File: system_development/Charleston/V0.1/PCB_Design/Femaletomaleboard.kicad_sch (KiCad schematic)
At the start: 5 parts, among them J1 DB25_Receptacle, J2 Screw_Terminal_01x12, J3 Screw_Terminal_01x12

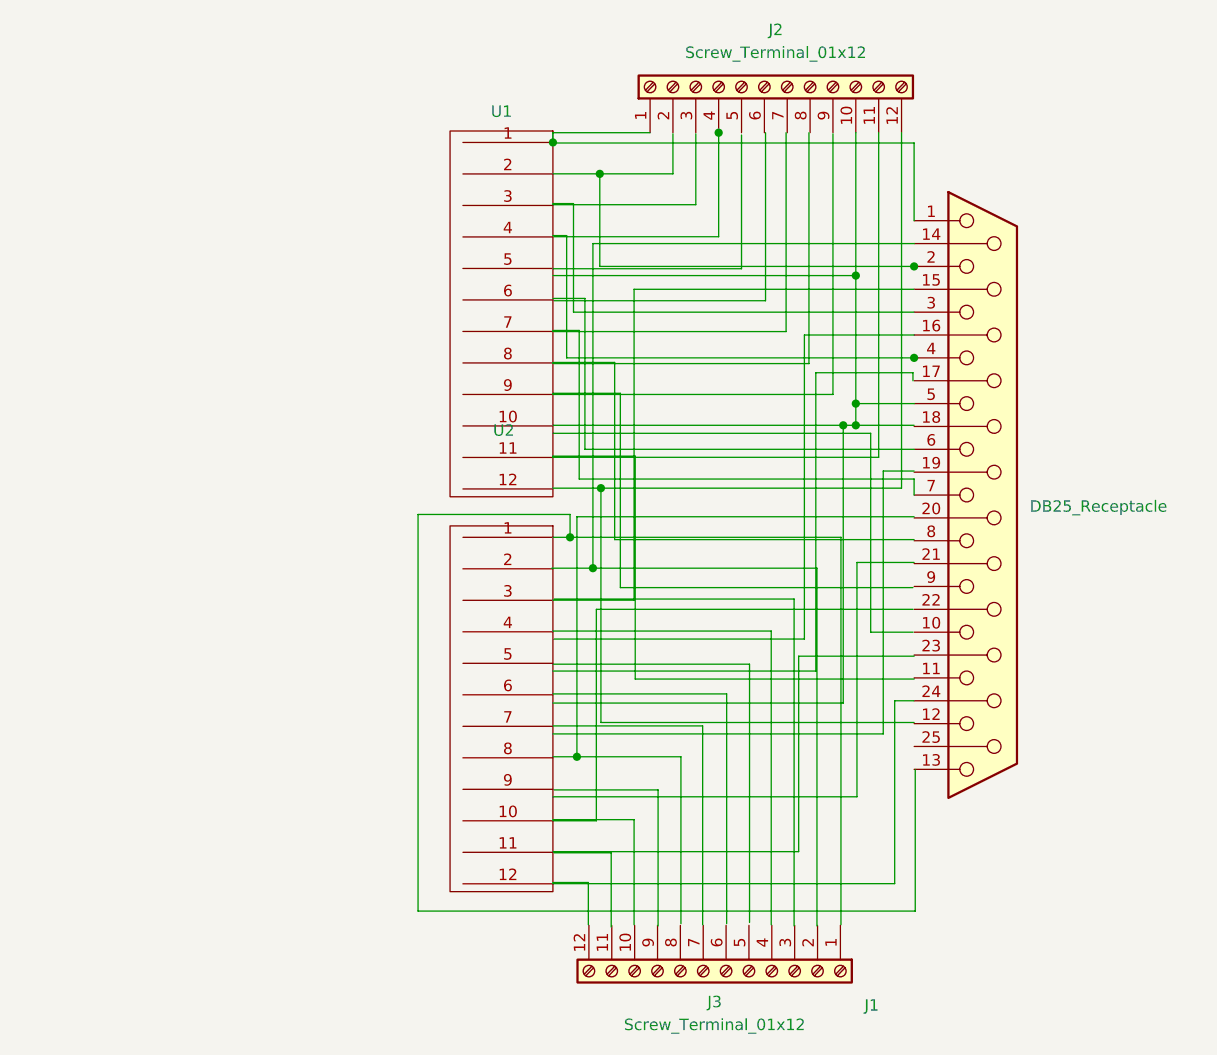
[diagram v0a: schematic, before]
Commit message: femaletomaleboard
4th times the charm
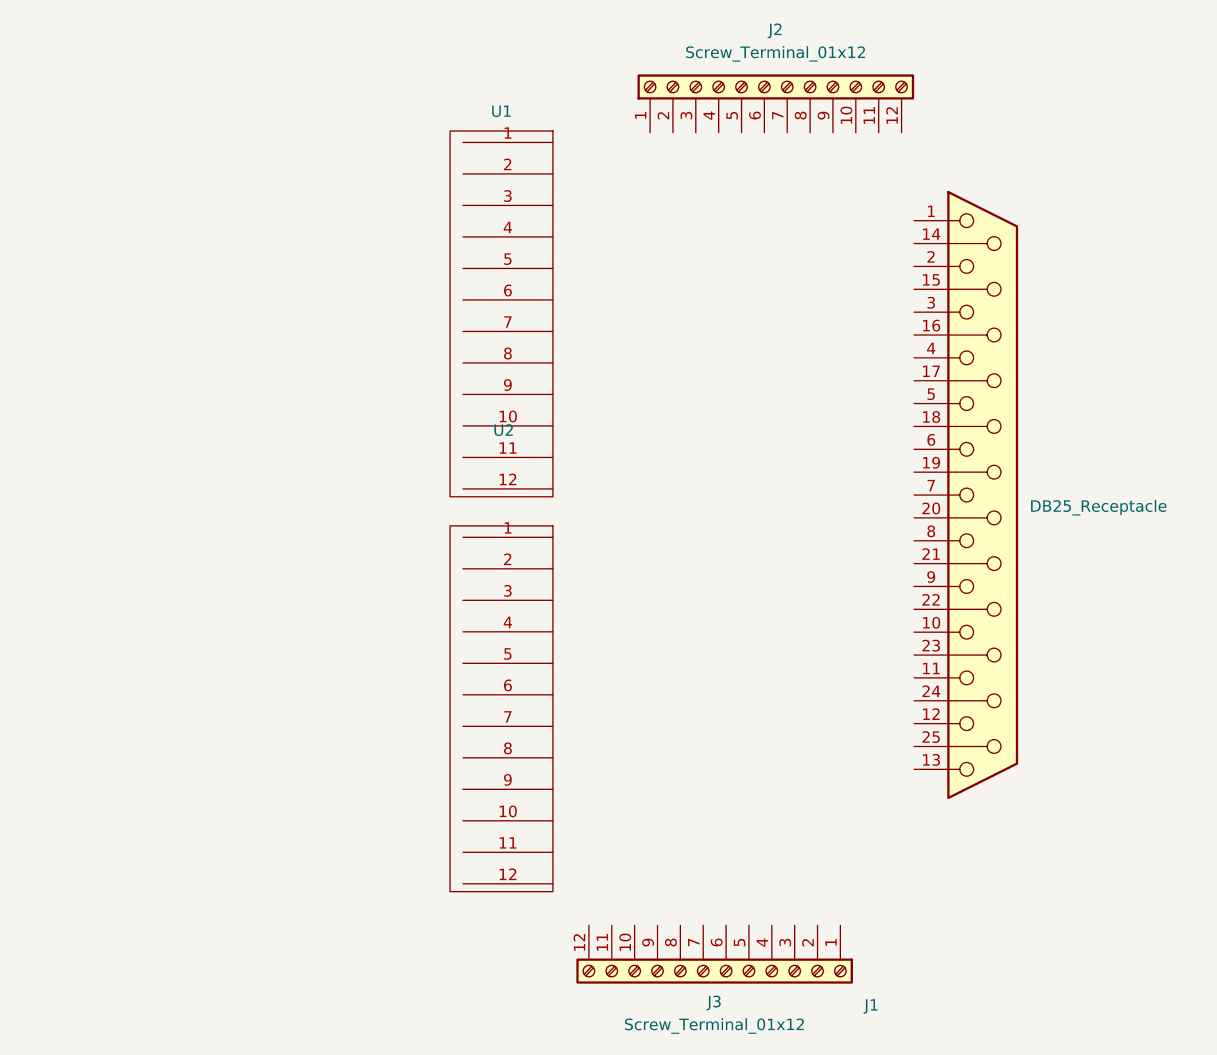
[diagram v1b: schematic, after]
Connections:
- net at J1.5: no longer J2.10 (Pin_10)
- now unconnected: J1.1, J2.1 (Pin_1), U1.1

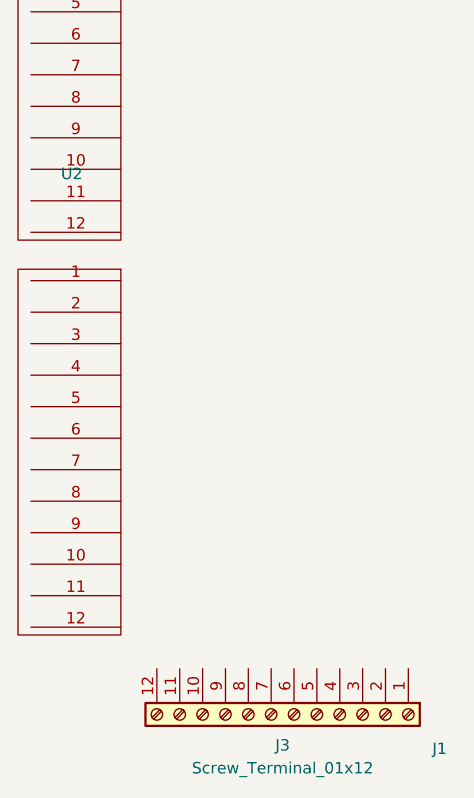
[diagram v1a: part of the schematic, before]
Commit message: updates
updates
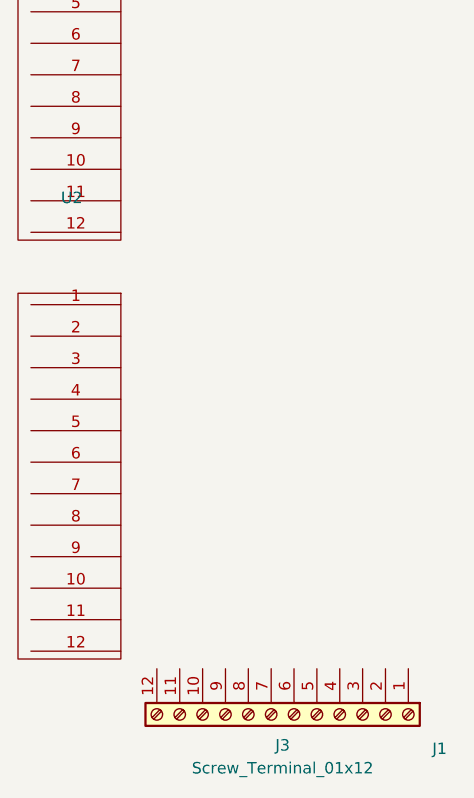
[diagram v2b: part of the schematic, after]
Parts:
- J1: symbol Connector:DB25_Receptacle -> libary_bms:DB25_Receptacle
- J2, J3: symbol Connector:Screw_Terminal_01x12 -> libary_bms:Screw_Terminal_01x12
- U1, U2: symbol Gold_Finger_connector:GoldFingerConnector -> libary_bms:GoldFingerConnector
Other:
- moved on the sheet: U2
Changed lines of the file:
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@@
 (kicad_sch (version 20230121) (generator eeschema)
   (paper "A4")
-  (symbol (lib_id "Connector:Screw_Terminal_01x12") (at 93.7895 114.7445 270) (unit 1)
+  (symbol (lib_id "libary_bms:Screw_Terminal_01x12") (at 93.7895 114.7445 270) (unit 1)
     (in_bom yes) (on_board yes) (dnp no) (fields_autoplaced)
     (property "Reference" "J3" (at 92.5195 118.1735 90)
@@
     )
   )
-  (symbol (lib_id "Gold_Finger_connector:GoldFingerConnector") (at 74.549 66.548 180) (unit 1)
+  (symbol (lib_id "libary_bms:GoldFingerConnector") (at 74.549 69.215 180) (unit 1)
     (in_bom yes) (on_board yes) (dnp no)
-    (property "Reference" "U2" (at 69.088 54.677 0)
+    (property "Reference" "U2" (at 69.088 57.344 0)
       (effects (font (size 1.27 1.27)))
     )
-    (property "Value" "~" (at 74.549 66.548 0)
+    (property "Value" "~" (at 74.549 69.215 0)
       (effects (font (size 1.27 1.27)))
     )
-    (property "Footprint" "" (at 74.549 66.548 0)
+    (property "Footprint" "" (at 74.549 69.215 0)
       (effects (font (size 1.27 1.27)) hide)
     )
-    (property "Datasheet" "" (at 74.549 66.548 0)
+    (property "Datasheet" "" (at 74.549 69.215 0)
       (effects (font (size 1.27 1.27)) hide)
     )
@@
     )
   )
-  (symbol (lib_id "Connector:DB25_Receptacle") (at 122.301 61.849 0) (unit 1)
+  (symbol (lib_id "libary_bms:DB25_Receptacle") (at 122.301 61.849 0) (unit 1)
     (in_bom yes) (on_board yes) (dnp no)
     (property "Reference" "J1" (at 109.1565 118.5545 0)
@@
     )
   )
-  (symbol (lib_id "Gold_Finger_connector:GoldFingerConnector") (at 74.549 22.673 180) (unit 1)
+  (symbol (lib_id "libary_bms:GoldFingerConnector") (at 74.549 22.673 180) (unit 1)
     (in_bom yes) (on_board yes) (dnp no)
     (property "Reference" "U1" (at 68.834 19.244 0)
@@
     )
   )
-  (symbol (lib_id "Connector:Screw_Terminal_01x12") (at 98.044 16.51 90) (unit 1)
+  (symbol (lib_id "libary_bms:Screw_Terminal_01x12") (at 98.044 16.51 90) (unit 1)
     (in_bom yes) (on_board yes) (dnp no) (fields_autoplaced)
     (property "Reference" "J2" (at 99.314 10.16 90)

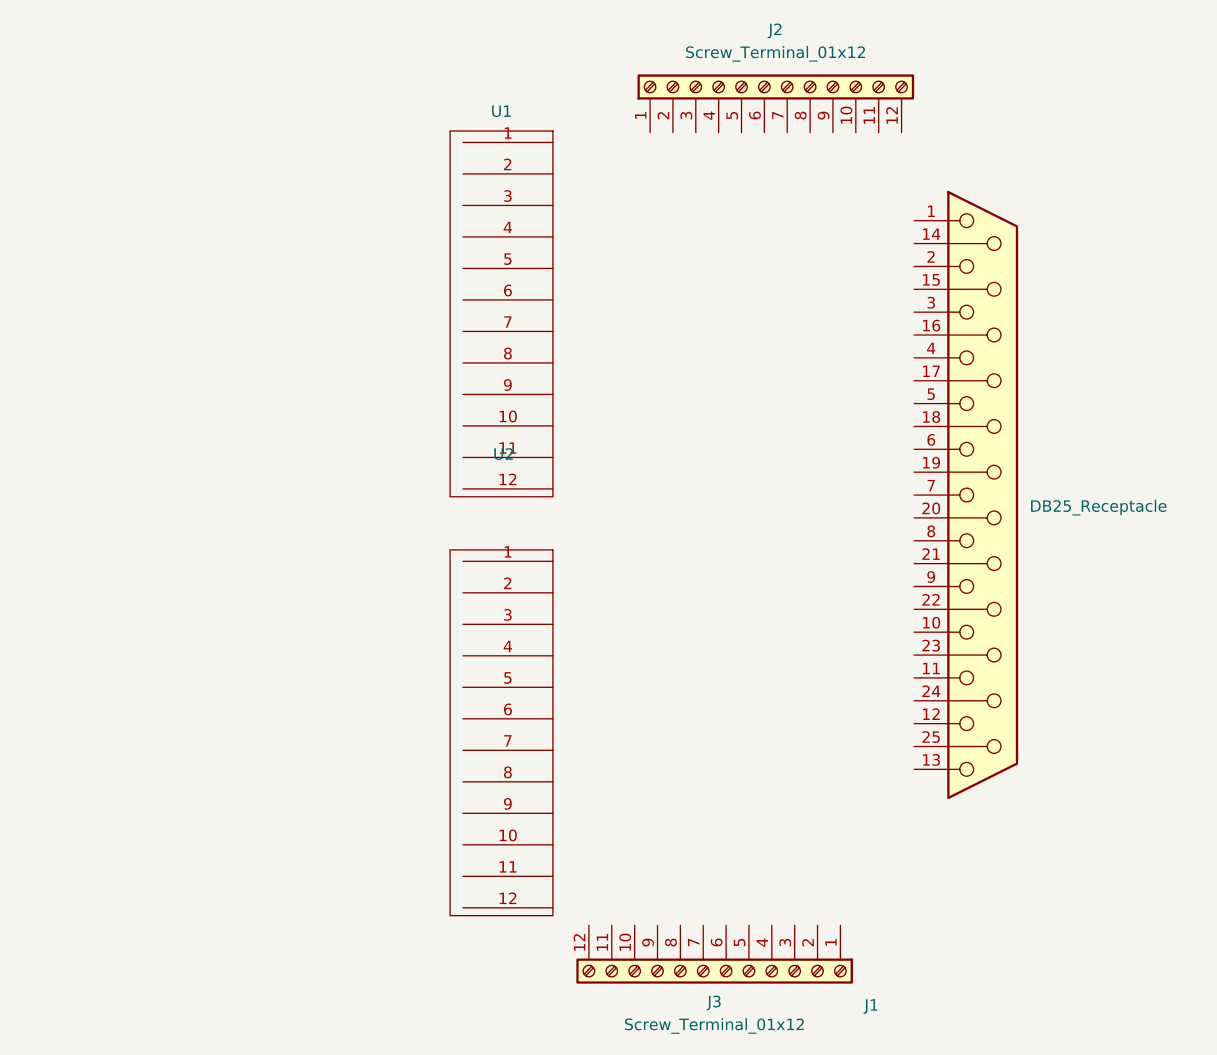
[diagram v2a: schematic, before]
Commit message: Assembled Libraries
Assembled Libraries
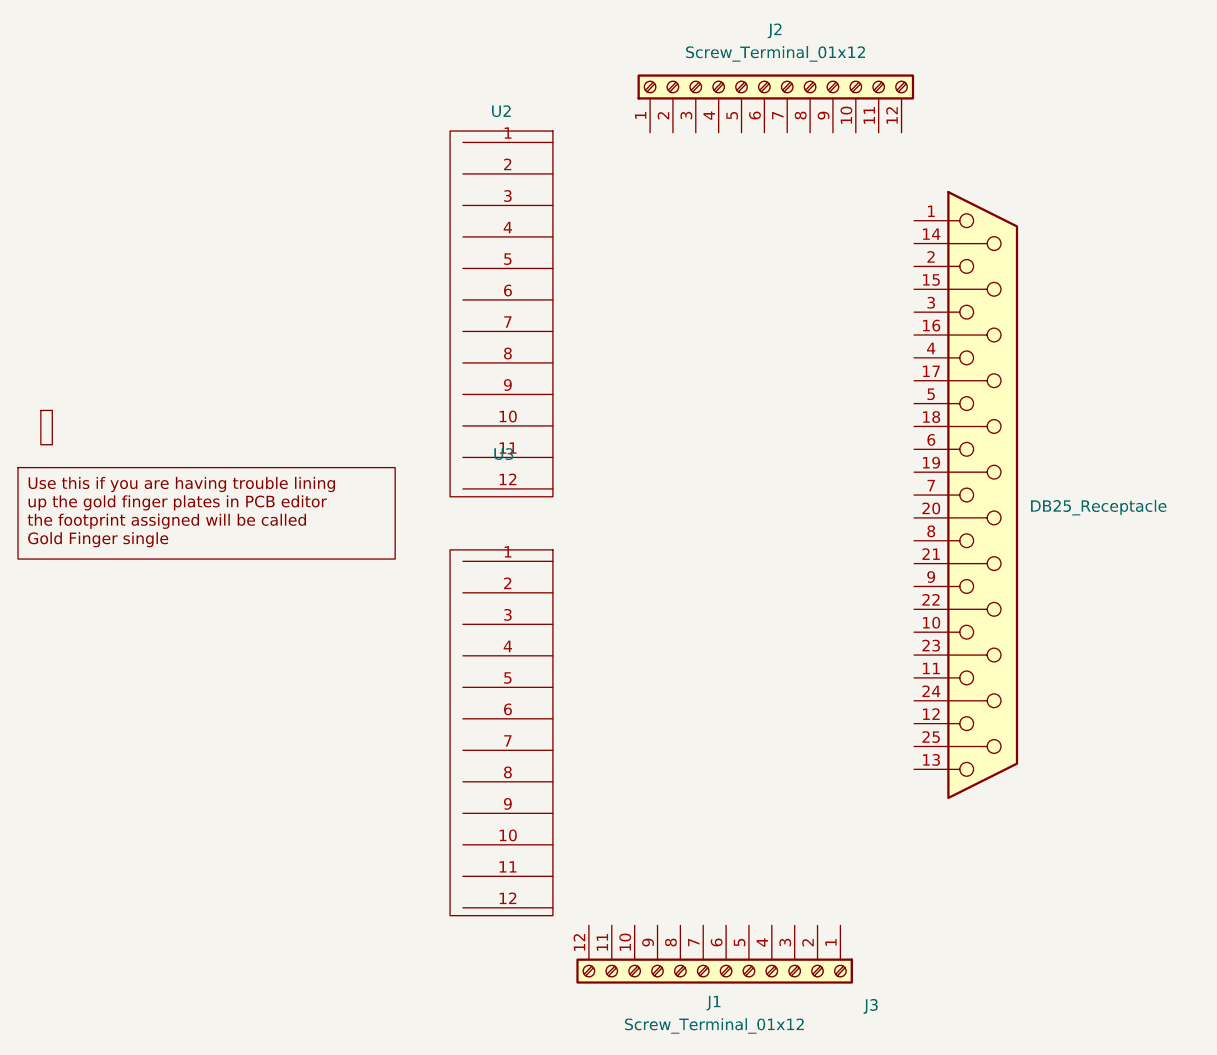
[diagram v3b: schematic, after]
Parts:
- added U1: ~, infnoise_goldfingers:Gold Finger single, symbol libary_bms:Goldfingersingle
- J1: renamed from J3; footprint (none) -> infnoise_goldfingers:Gold Finger single
- J2: footprint (none) -> TerminalBlock_Altech:Altech_AK300_1x12_P5.00mm_45-Degree
- U2: renamed from U1; footprint (none) -> infnoise_goldfingers:Gold Finger PCB
- U3: renamed from U2; footprint (none) -> infnoise_goldfingers:Gold Finger PCB
- renumbered J1 to J3
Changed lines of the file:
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@@
   (symbol (lib_id "libary_bms:Screw_Terminal_01x12") (at 93.7895 114.7445 270) (unit 1)
     (in_bom yes) (on_board yes) (dnp no) (fields_autoplaced)
-    (property "Reference" "J3" (at 92.5195 118.1735 90)
+    (property "Reference" "J1" (at 92.5195 118.1735 90)
       (effects (font (size 1.27 1.27)))
     )
@@
       (effects (font (size 1.27 1.27)))
     )
-    (property "Footprint" "" (at 93.7895 114.7445 0)
+    (property "Footprint" "infnoise_goldfingers:Gold Finger single" (at 93.7895 114.7445 0)
       (effects (font (size 1.27 1.27)) hide)
     )
@@
       (project "Femaletomaleboard"
         (path "/8dcdbe00-6c4e-43b9-b640-476052a1e30f"
-          (reference "J3") (unit 1)
+          (reference "J1") (unit 1)
         )
       )
@@
   (symbol (lib_id "libary_bms:GoldFingerConnector") (at 74.549 69.215 180) (unit 1)
     (in_bom yes) (on_board yes) (dnp no)
-    (property "Reference" "U2" (at 69.088 57.344 0)
+    (property "Reference" "U3" (at 69.088 57.344 0)
       (effects (font (size 1.27 1.27)))
     )
@@
       (effects (font (size 1.27 1.27)))
     )
-    (property "Footprint" "" (at 74.549 69.215 0)
+    (property "Footprint" "infnoise_goldfingers:Gold Finger PCB" (at 74.549 69.215 0)
       (effects (font (size 1.27 1.27)) hide)
     )
@@
       (project "Femaletomaleboard"
         (path "/8dcdbe00-6c4e-43b9-b640-476052a1e30f"
-          (reference "U2") (unit 1)
+          (reference "U3") (unit 1)
+        )
+      )
+    )
+  )
+  (symbol (lib_id "libary_bms:Goldfingersingle") (at 16.383 53.721 0) (unit 1)
+    (in_bom yes) (on_board yes) (dnp no) (fields_autoplaced)
+    (property "Reference" "U1" (at 20.193 54.356 0)
+      (effects (font (size 1.27 1.27)) (justify left) hide)
+    )
+    (property "Value" "~" (at 16.383 53.721 0)
+      (effects (font (size 1.27 1.27)))
+    )
+    (property "Footprint" "infnoise_goldfingers:Gold Finger single" (at 16.383 53.721 0)
+      (effects (font (size 1.27 1.27)) hide)
+    )
+    (property "Datasheet" "" (at 16.383 53.721 0)
+      (effects (font (size 1.27 1.27)) hide)
+    )
+    (instances
+      (project "Femaletomaleboard"
+        (path "/8dcdbe00-6c4e-43b9-b640-476052a1e30f"
+          (reference "U1") (unit 1)
         )
       )
@@
   (symbol (lib_id "libary_bms:DB25_Receptacle") (at 122.301 61.849 0) (unit 1)
     (in_bom yes) (on_board yes) (dnp no)
-    (property "Reference" "J1" (at 109.1565 118.5545 0)
+    (property "Reference" "J3" (at 109.1565 118.5545 0)
       (effects (font (size 1.27 1.27)) (justify left))
     )
@@
       (project "Femaletomaleboard"
         (path "/8dcdbe00-6c4e-43b9-b640-476052a1e30f"
-          (reference "J1") (unit 1)
+          (reference "J3") (unit 1)
         )
       )
@@
   (symbol (lib_id "libary_bms:GoldFingerConnector") (at 74.549 22.673 180) (unit 1)
     (in_bom yes) (on_board yes) (dnp no)
-    (property "Reference" "U1" (at 68.834 19.244 0)
+    (property "Reference" "U2" (at 68.834 19.244 0)
       (effects (font (size 1.27 1.27)))
     )
@@
       (effects (font (size 1.27 1.27)))
     )
-    (property "Footprint" "" (at 74.549 22.673 0)
+    (property "Footprint" "infnoise_goldfingers:Gold Finger PCB" (at 74.549 22.673 0)
       (effects (font (size 1.27 1.27)) hide)
     )
@@
       (project "Femaletomaleboard"
         (path "/8dcdbe00-6c4e-43b9-b640-476052a1e30f"
-          (reference "U1") (unit 1)
+          (reference "U2") (unit 1)
         )
       )
@@
       (effects (font (size 1.27 1.27)))
     )
-    (property "Footprint" "" (at 98.044 16.51 0)
+    (property "Footprint" "TerminalBlock_Altech:Altech_AK300_1x12_P5.00mm_45-Degree" (at 98.044 16.51 0)
       (effects (font (size 1.27 1.27)) hide)
     )
